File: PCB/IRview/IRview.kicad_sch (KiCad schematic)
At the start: 18 parts, among them J1 Conn_01x05_Pin, J2 Conn_01x08_Pin, J4 Conn_01x02_Pin, J5 Conn_01x11_Pin, SW1 SW_Push, SW2 SW_Push, SW3 SW_Push, SW4 SW_Push, SW5 SW_Push, SW6 SW_Push, U1 ESP32-WROOM-32E-R2, U2 AMS1117-3.3

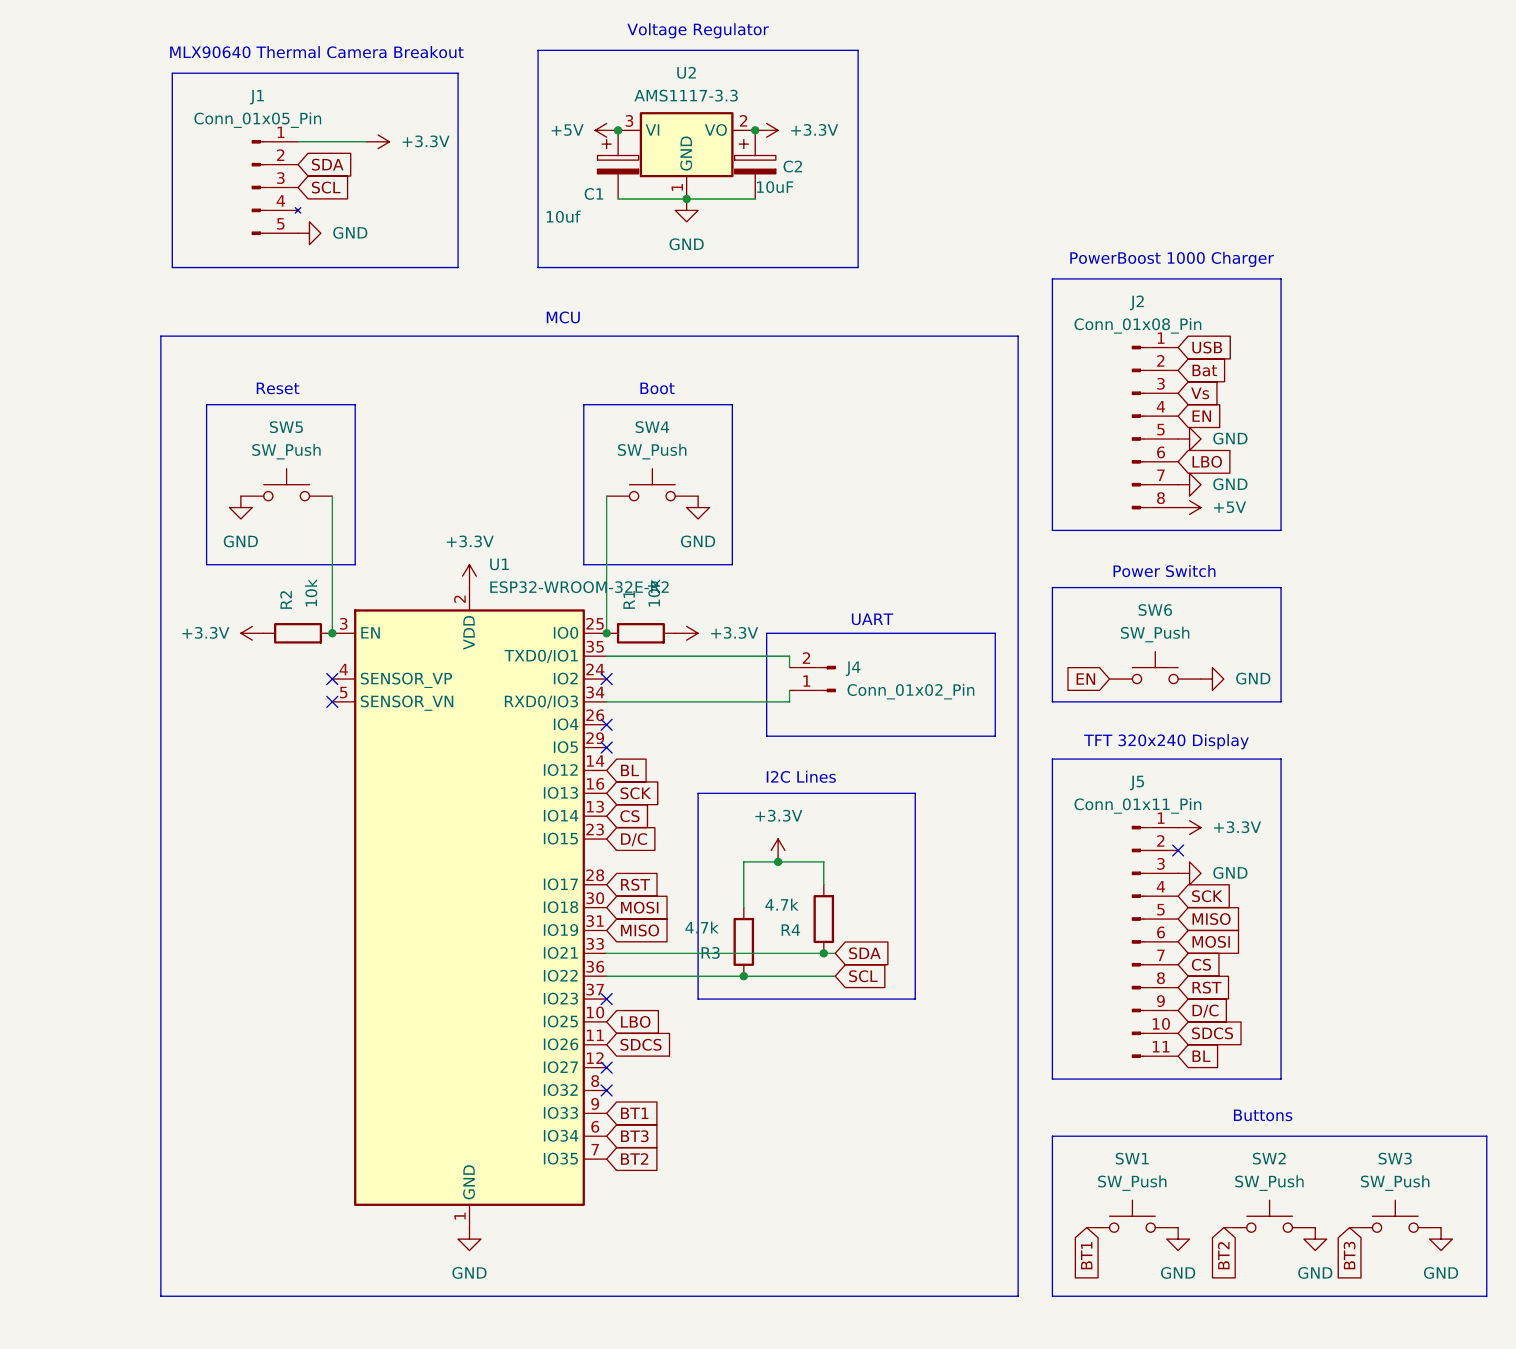
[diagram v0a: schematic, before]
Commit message: change esp and rewire
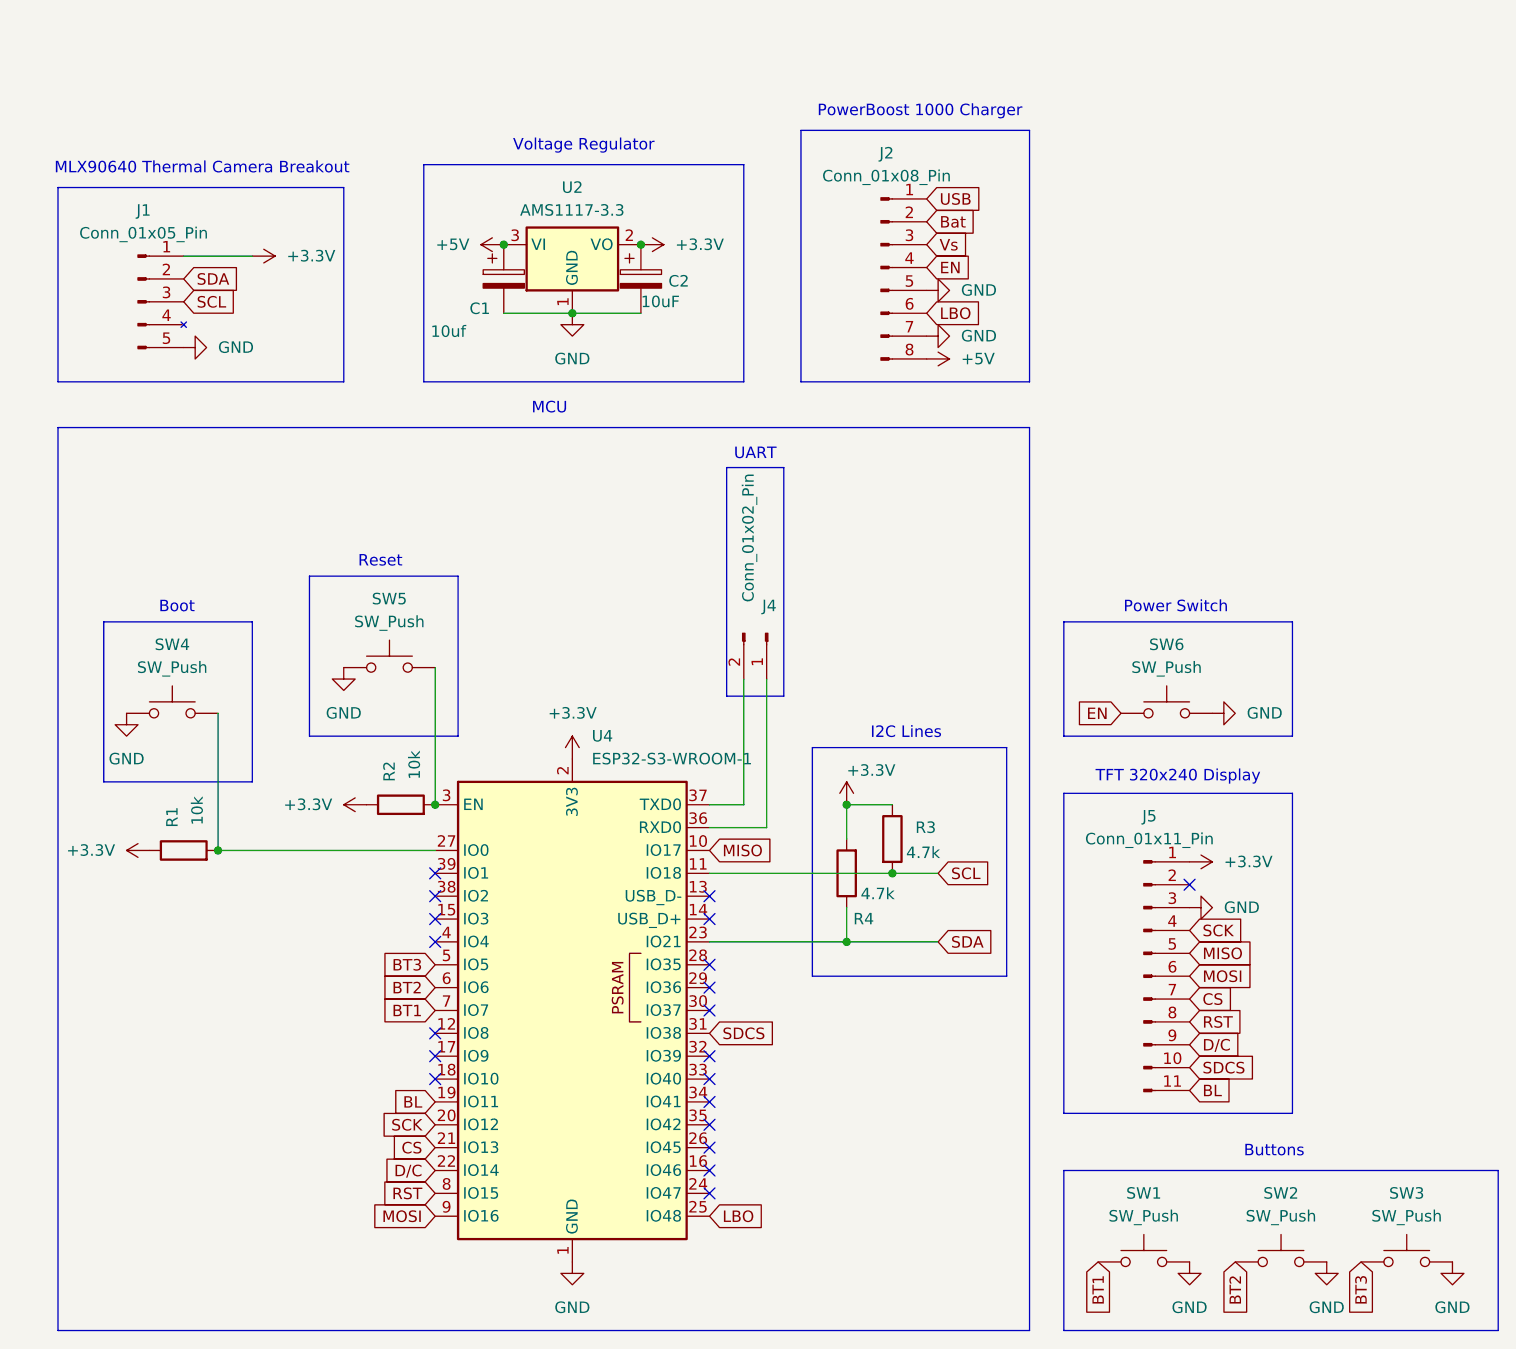
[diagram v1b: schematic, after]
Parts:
- removed U1: ESP32-WROOM-32E-R2, RF_Module:ESP32-WROOM-32D, symbol RF_Module:ESP32-WROOM-32E-R2
- added U4: ESP32-S3-WROOM-1, RF_Module:ESP32-S3-WROOM-1, symbol RF_Module:ESP32-S3-WROOM-1
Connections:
- net +3.3V: now also R1.1, R3.1, U4.2 (3V3); no longer R1.2, R3.2
- net BL: now also U4.19 (IO11)
- net BT1: now also U4.7 (IO7)
- net BT2: now also U4.6 (IO6)
- net BT3: now also U4.5 (IO5)
- net CS: now also U4.21 (IO13)
- net D/C: now also U4.22 (IO14)
- net GND: now also SW4.1, U4.1 (GND), U4.40 (GND), U4.41 (GND); no longer SW4.2
- net LBO: now also U4.25 (IO48)
- net MISO: now also U4.10 (IO17)
- net MOSI: now also U4.9 (IO16)
- net RST: now also U4.8 (IO15)
- net SCK: now also U4.20 (IO12)
- net SCL: now also R3.2, U4.11 (IO18); no longer R3.1
- net SDA: now also U4.23 (IO21)
- net SDCS: now also U4.31 (IO38)
- net at R2.2, SW5.2: now also U4.3 (EN)
- net at J4.1 (Pin_1): now also U4.36 (RXD0)
- net at J4.2 (Pin_2): now also U4.37 (TXD0)
- new net: R1.2, SW4.2, U4.27 (IO0)
- no-connect marks 9 -> 20
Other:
- moved on the sheet: C1, C2, J1, J2, J5, SW1, SW2, SW3, SW6, U2
